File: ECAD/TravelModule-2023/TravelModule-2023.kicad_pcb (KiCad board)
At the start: 2 copper layers, 2 parts

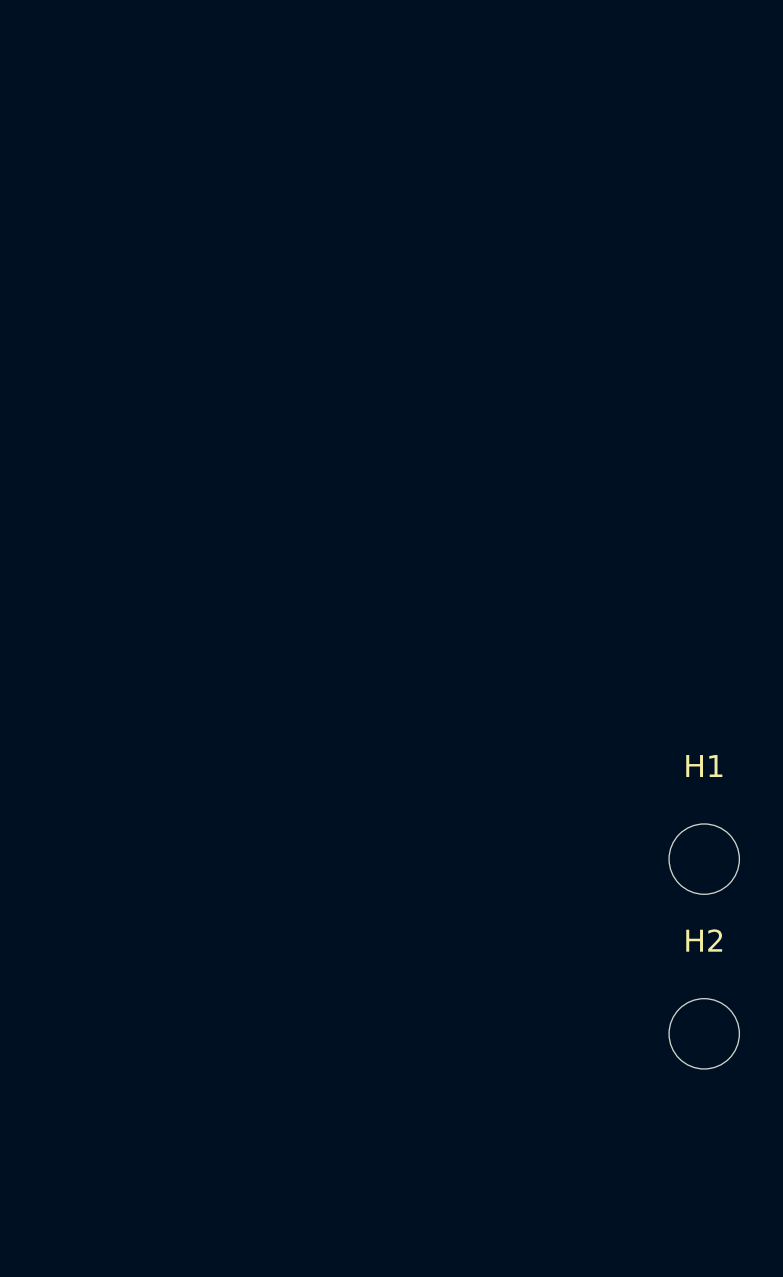
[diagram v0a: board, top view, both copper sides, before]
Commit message: Update deplacmentSensor
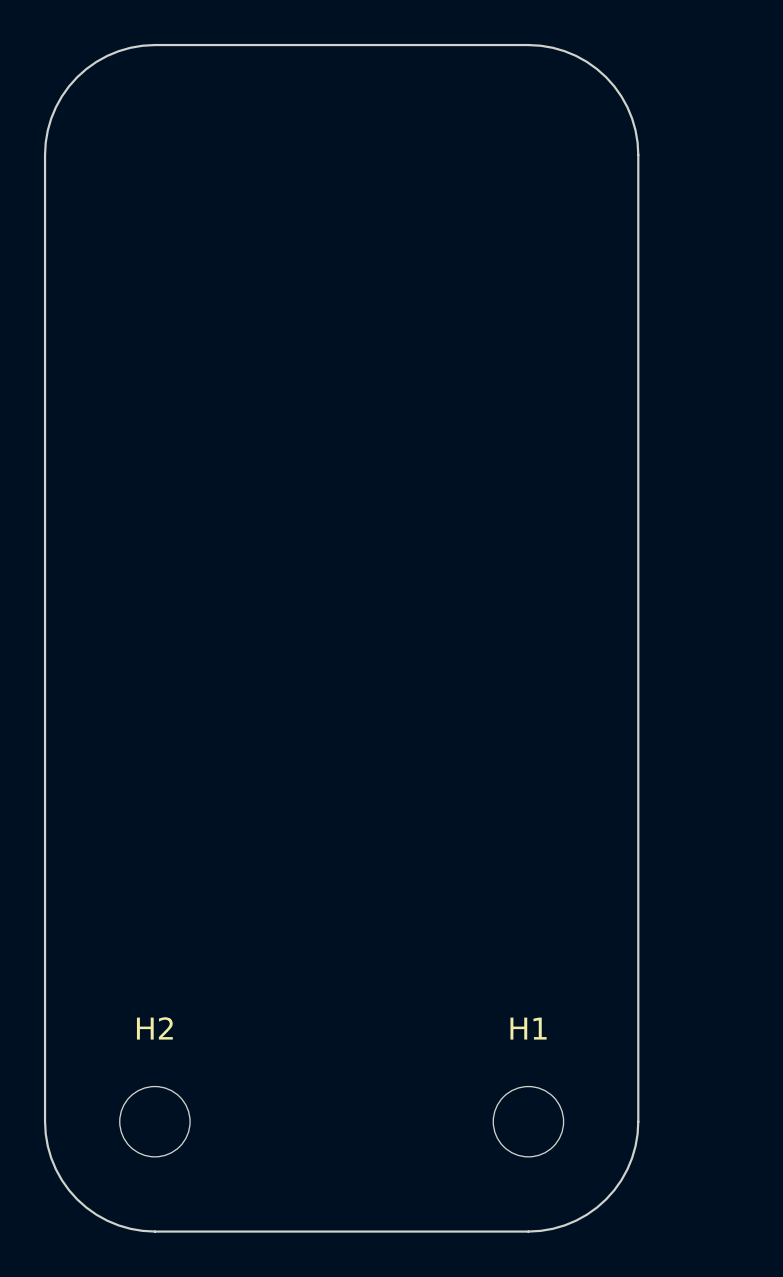
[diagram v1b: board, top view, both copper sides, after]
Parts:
- moved H2 25.3 mm to (113.0, 80.0)
- moved H1 14.4 mm to (130.0, 80.0)
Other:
- board outline added: 27 x 54 mm
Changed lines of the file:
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@@
   (net 0 "")
   (footprint "MountingHole:MountingHole_3.2mm_M3" (layer "F.Cu")
-    (at 138 76)
+    (at 113 80)
     (descr "Mounting Hole 3.2mm, no annular, M3")
     (tags "mounting hole 3.2mm no annular m3")
@@
   )
   (footprint "MountingHole:MountingHole_3.2mm_M3" (layer "F.Cu")
-    (at 138 68.05)
+    (at 130 80)
     (descr "Mounting Hole 3.2mm, no annular, M3")
     (tags "mounting hole 3.2mm no annular m3")
@@
     (pad "" np_thru_hole circle (at 0 0) (size 3.2 3.2) (drill 3.2) (layers "*.Cu" "*.Mask"))
   )
+  (gr_line (start 113 85) (end 130 85)
+    (stroke (width 0.1) (type default)) (layer "Edge.Cuts"))
+  (gr_arc (start 113 85) (mid 109.464466 83.535534) (end 108 80)
+    (stroke (width 0.1) (type default)) (layer "Edge.Cuts"))
+  (gr_line (start 108 36) (end 108 80)
+    (stroke (width 0.1) (type default)) (layer "Edge.Cuts"))
+  (gr_arc (start 130 31) (mid 133.535534 32.464466) (end 135 36)
+    (stroke (width 0.1) (type default)) (layer "Edge.Cuts"))
+  (gr_line (start 113 31) (end 130 31)
+    (stroke (width 0.1) (type default)) (layer "Edge.Cuts"))
+  (gr_arc (start 135 80) (mid 133.535534 83.535534) (end 130 85)
+    (stroke (width 0.1) (type default)) (layer "Edge.Cuts"))
+  (gr_line (start 135 80) (end 135 36)
+    (stroke (width 0.1) (type default)) (layer "Edge.Cuts"))
+  (gr_arc (start 108 36) (mid 109.464466 32.464466) (end 113 31)
+    (stroke (width 0.1) (type default)) (layer "Edge.Cuts"))
+  (dimension (type aligned) (layer "User.1")
+    (pts (xy 108 80) (xy 135 80))
+    (height 14)
+    (gr_text "27,0000 mm" (at 121.5 92.85) (layer "User.1")
+      (effects (font (size 1 1) (thickness 0.15)))
+    )
+    (format (prefix "") (suffix "") (units 3) (units_format 1) (precision 4))
+    (style (thickness 0.15) (arrow_length 1.27) (text_position_mode 0) (extension_height 0.58642) (extension_offset 0.5) keep_text_aligned)
+  )
+  (dimension (type aligned) (layer "User.1")
+    (pts (xy 130 80) (xy 113 80))
+    (height -11)
+    (gr_text "17,0000 mm" (at 121.5 89.85) (layer "User.1")
+      (effects (font (size 1 1) (thickness 0.15)))
+    )
+    (format (prefix "") (suffix "") (units 3) (units_format 1) (precision 4))
+    (style (thickness 0.15) (arrow_length 1.27) (text_position_mode 0) (extension_height 0.58642) (extension_offset 0.5) keep_text_aligned)
+  )
 )
